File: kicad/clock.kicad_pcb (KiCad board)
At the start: 4 copper layers, 110 x 110 mm, 187 parts, among them J1 USB4160-03-0230-C, J10 Knob: EM14 enc+SW (top face), J11 Radio-off toggle (rear), J12 NeoPixel ext (5V/DATA/GND, po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, J2 PROG, J3 Speaker DMA58-4 (4R), J6 DM3AT-SF-PEJM5, J7 Sensor board (BME688+TSL2591+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, J9 Wake COB 12V (warm+cool), M1 X40.879, Q1 2N7002, Q2 AO3401A, Q3 2N7002, Q4 AO3401A, Q6 AO3400A, Q7 AO3400A, Q8 2N7002, Q9 AO3401A, SW1 RESET, SW2 BOOT, U1 CH224K, U10 LTC4412ES6, U11 TB6612FNG, U12 TB6612FNG, U13 MCP23017, U14 QRE1113GR, U15 SN74AHCT1G125, U16 USBLC6-2SC6, U2 LT3652EMSE, U3 HY2111-GB, U4 AOSD32334C, U5 TPS61023, U6 TLV62569DBVR, U7 TPS55340PWPR, U8 ESP32-S3-WROOM-1-N16R8, U9 TAS5760MDAPR, Y1 32.768kHz

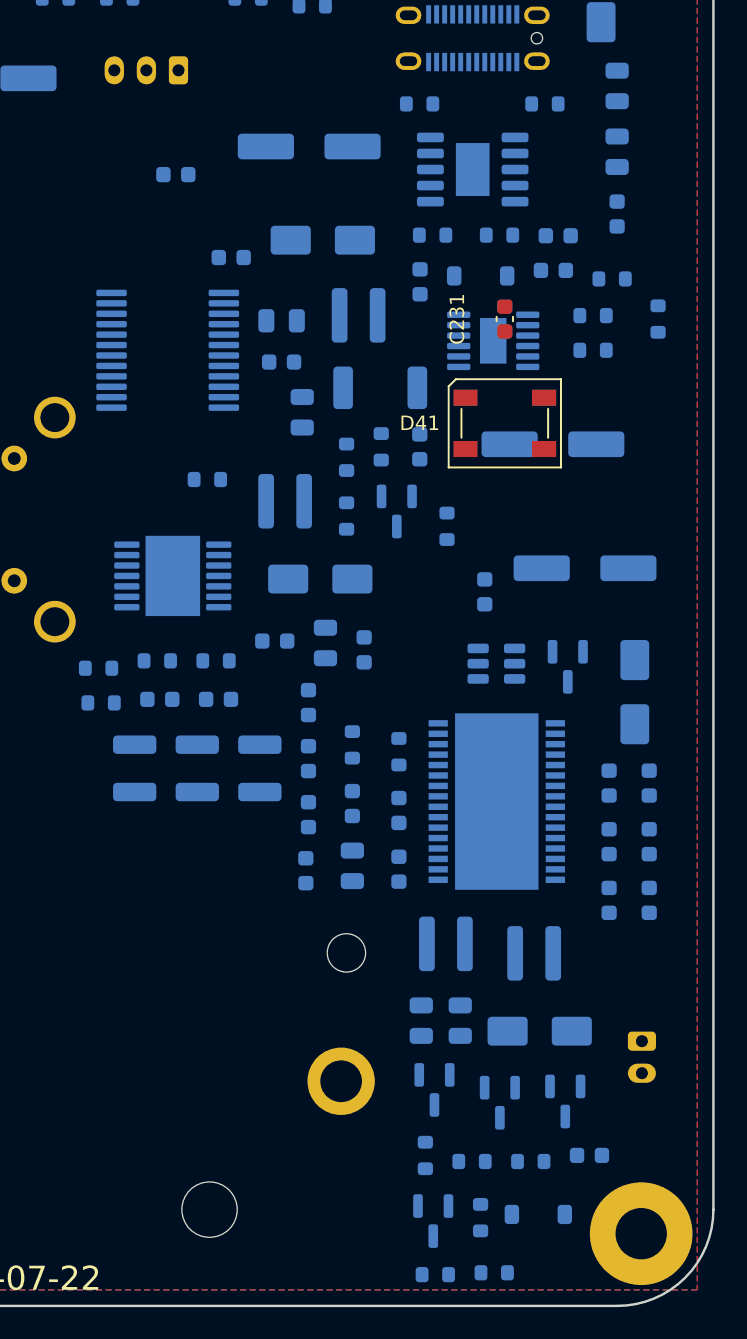
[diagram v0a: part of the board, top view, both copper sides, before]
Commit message: schematic verification pass
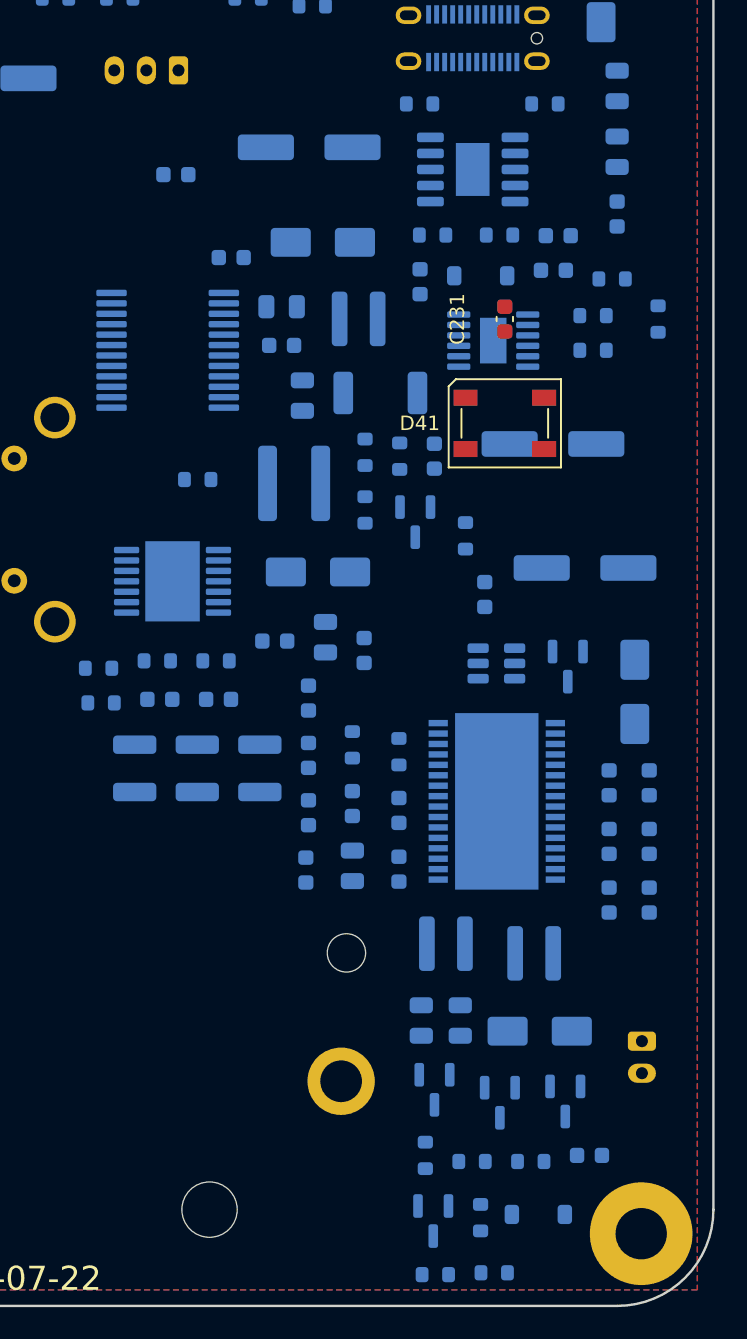
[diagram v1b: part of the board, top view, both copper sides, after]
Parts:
- D30: value SS34 -> B340A
- L4: footprint Inductor_SMD:L_Coilcraft_XAL4030-XXX -> Inductor_SMD:L_Coilcraft_XAL5050-XXX
- moved Q1 1.33 mm to (91.4, 61.2)
- moved R24 1.29 mm to (94.5, 62.0)
- moved R15 1.29 mm to (90.4, 57.0)
- moved L4 1.25 mm to (83.9, 58.7)
- moved R16 1.21 mm to (88.3, 60.4)
- moved R14 1.19 mm to (88.3, 56.8)
- moved C105 1.08 mm to (92.6, 57.0)
- moved C106 1.04 mm to (84.4, 53.3)
- moved C201 1.04 mm to (83.1, 50.1)
- moved C200 0.88 mm to (83.1, 47.7)
- moved R44 0.60 mm to (77.9, 58.5)
- moved D20 0.46 mm to (85.4, 64.3)
- moved C127 0.36 mm to (85.8, 68.3)
- moved U7 0.34 mm to (76.3, 64.8)
- moved R18 0.32 mm to (89.2, 53.1)
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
